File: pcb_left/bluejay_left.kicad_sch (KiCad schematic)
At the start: 20 parts, among them J1 SJ-43514, SW1A KEYSW, U1 ATmega328P-PU, Y1 16MHz

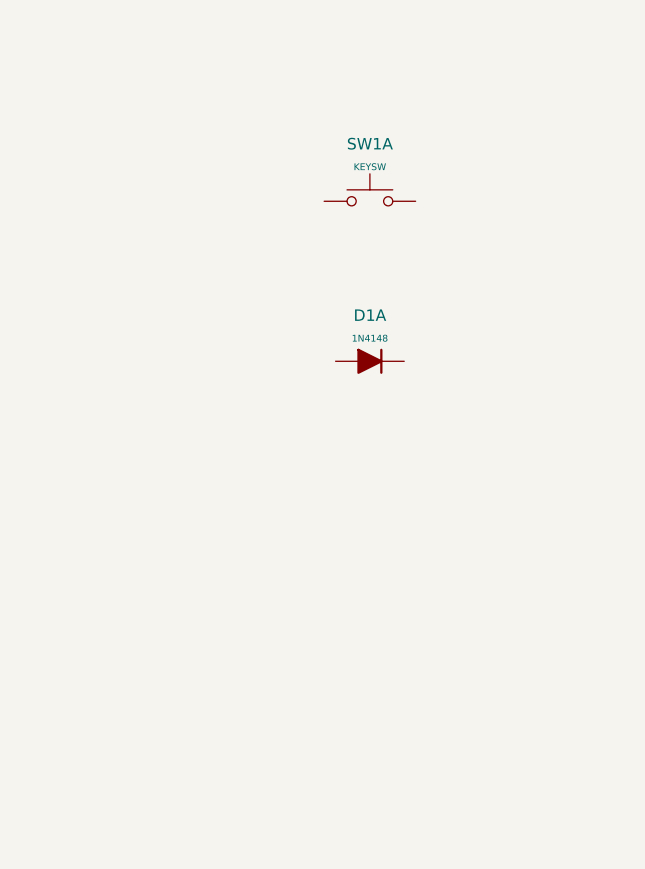
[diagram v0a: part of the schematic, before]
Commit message: Further progress with left hand schematic
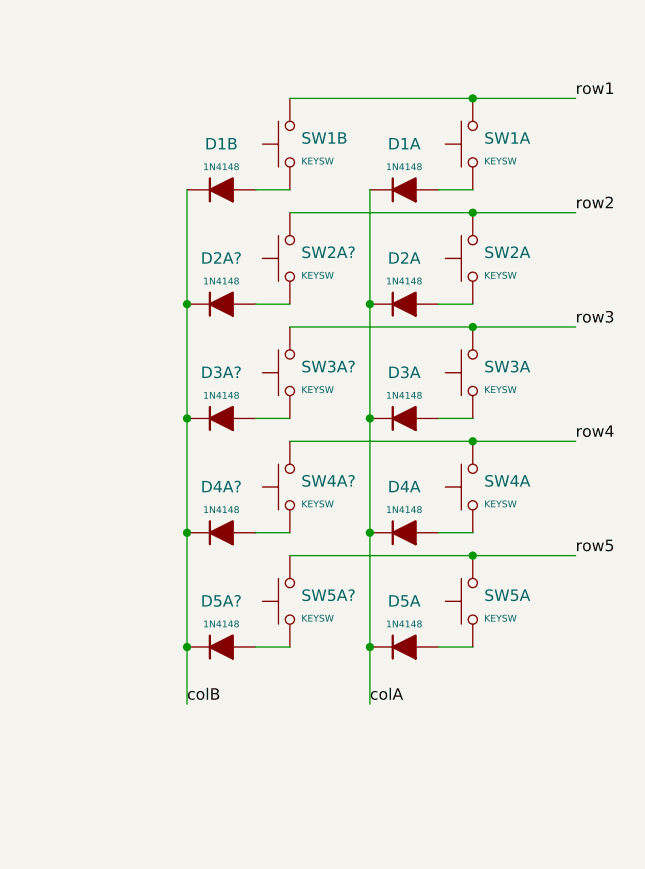
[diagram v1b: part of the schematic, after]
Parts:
- added D1B, D2A, D2A?, D3A, D3A?, D4A, D4A?, D5A, D5A?: 1N4148, Diode_THT_AKL:D_DO-35_SOD27_P7.62mm_Horizontal, symbol Diode_AKL:1N4148
- added SW1B, SW2A, SW2A?, SW3A, SW3A?, SW4A, SW4A?, SW5A, SW5A?: KEYSW, symbol BlueJaySymbolLibrary:Switch_SW_Push
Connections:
- net colA: now reaches D1A.1 (K)
- net colA: now also D2A.1 (K), D3A.1 (K), D4A.1 (K), D5A.1 (K)
- net at D1A.2 (A): now also SW1A.1
- net row1: now reaches SW1A.2
- net row1: now also SW1B.2
- new net: D4A.2 (A), SW4A.1
- new net: D2A.2 (A), SW2A.1
- new net: D3A?.2 (A), SW3A?.1
- new net: D2A?.2 (A), SW2A?.1
- new net: D4A?.2 (A), SW4A?.1
- new net: D1B.2 (A), SW1B.1
- new net: D5A?.2 (A), SW5A?.1
- new net: D3A.2 (A), SW3A.1
- new net: D5A.2 (A), SW5A.1
- new net colB: D1B.1 (K), D2A?.1 (K), D3A?.1 (K), D4A?.1 (K), D5A?.1 (K)
- new net row2: SW2A.2, SW2A?.2
- new net row3: SW3A.2, SW3A?.2
- new net row4: SW4A.2, SW4A?.2
- new net row5: SW5A.2, SW5A?.2
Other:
- moved on the sheet: D1A, SW1A
